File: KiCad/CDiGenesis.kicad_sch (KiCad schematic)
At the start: 7 parts, among them J1 Genesis, J2 CDi, J3 Conn_01x03, U1 ATtiny1616-M

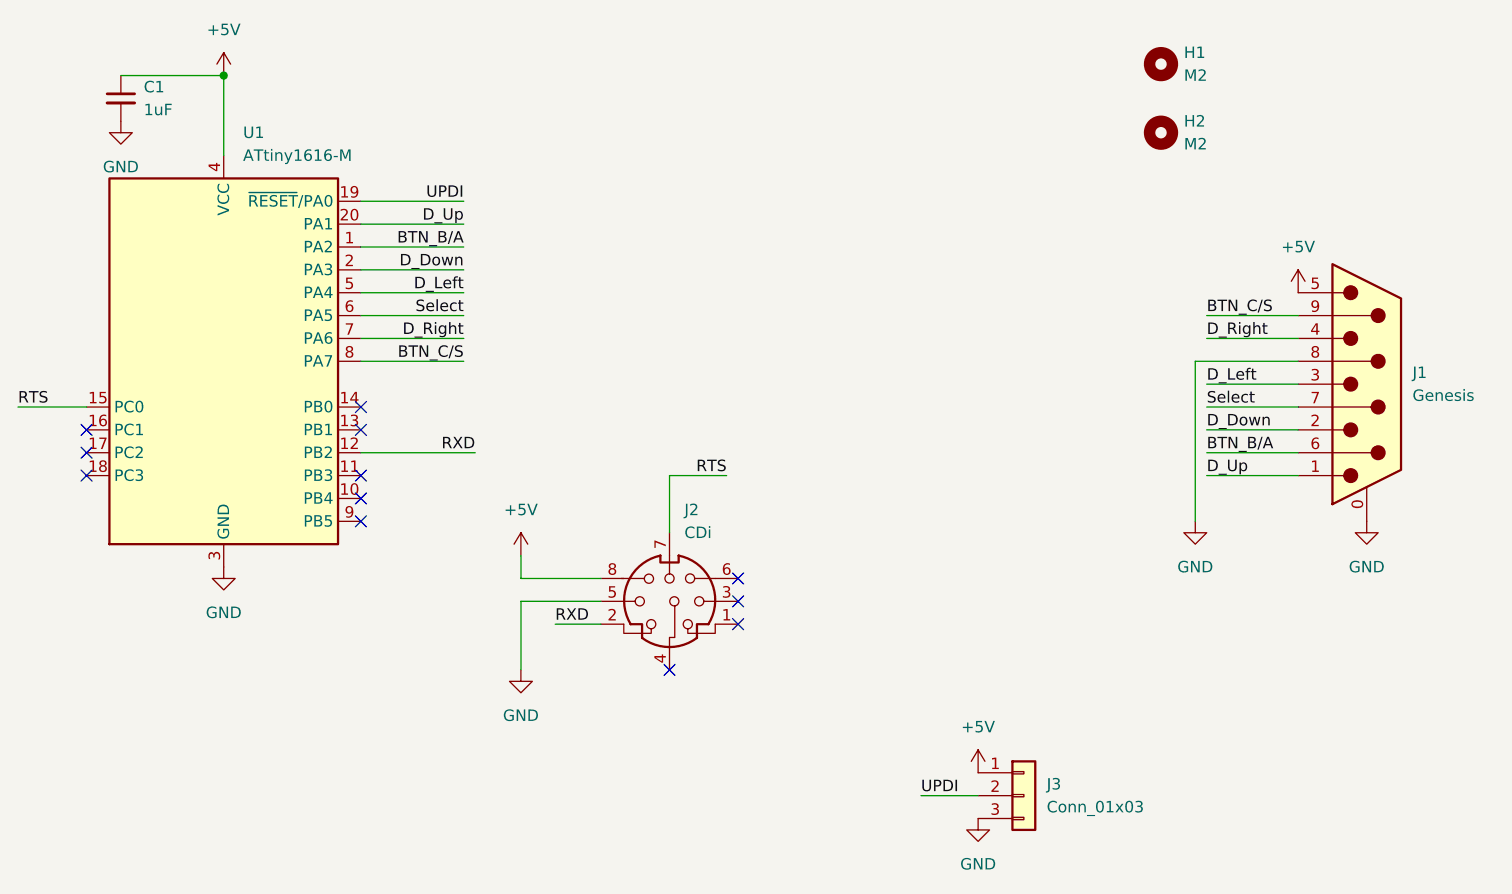
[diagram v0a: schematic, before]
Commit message: Effectively finalise code, remove SELECT nonsense
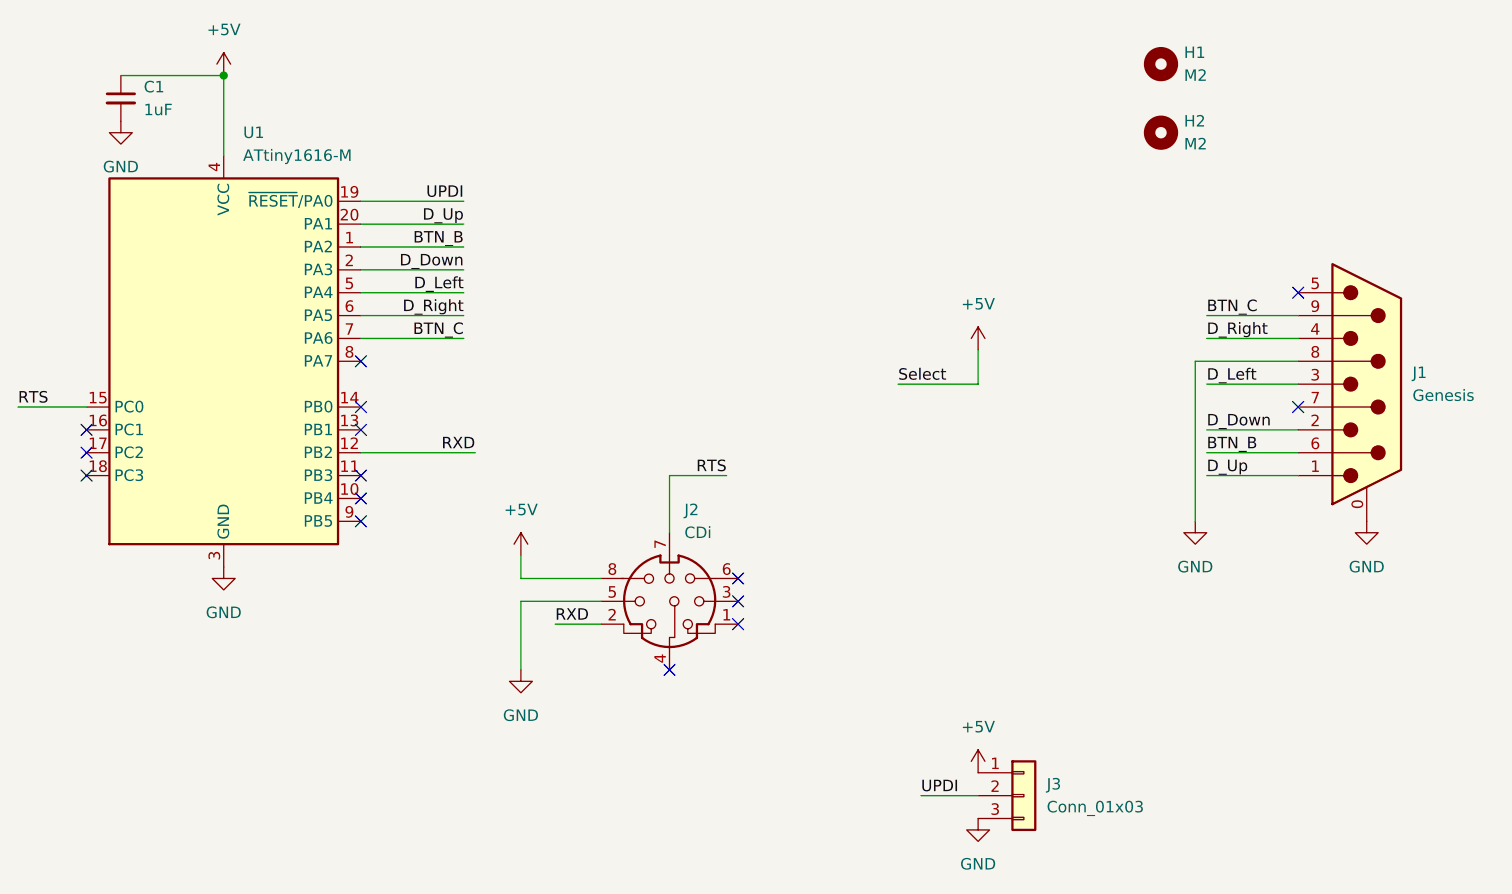
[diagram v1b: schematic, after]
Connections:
- net +5V: no longer J1.5
- net D_Right: now also U1.6 (PA5); no longer U1.7 (PA6)
- net BTN_B/A renamed BTN_B
- net BTN_C/S: no longer names the net of U1.8 (PA7)
- net BTN_C/S: no longer J1.9
- net Select: no longer names the net of J1.7
- net Select: no longer U1.6 (PA5)
- new net BTN_C: J1.9, U1.7 (PA6)
- no-connect marks 12 -> 15

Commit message: Revert PCB changes, will modify code
This reverts commit 0f8f6d9ed579b1546b77e135067905f4b0f0e6bf.
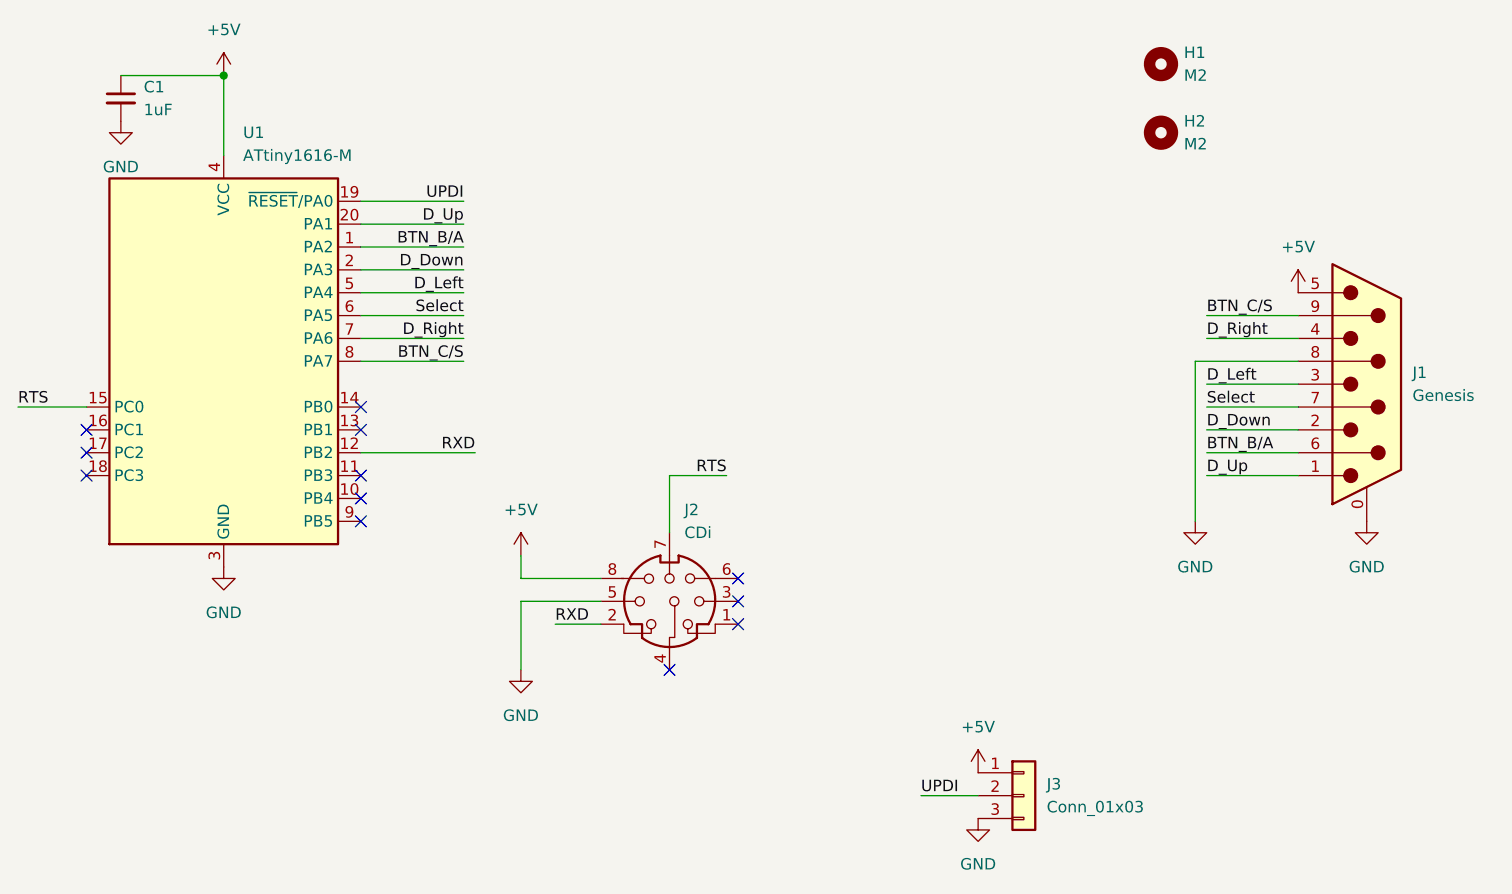
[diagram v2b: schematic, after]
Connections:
- net +5V: now also J1.5
- net D_Right: now also U1.7 (PA6); no longer U1.6 (PA5)
- net Select: now reaches J1.7
- net Select: now also U1.6 (PA5)
- net BTN_C/S: now reaches U1.8 (PA7)
- net BTN_C/S: now also J1.9
- net BTN_B renamed BTN_B/A
- removed net BTN_C: J1.9, U1.7 (PA6)
- no-connect marks 15 -> 12
